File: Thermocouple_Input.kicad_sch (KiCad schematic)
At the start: 9 parts, among them J7 K-TYPE THERMOCOUPLE, U11 MAX31856

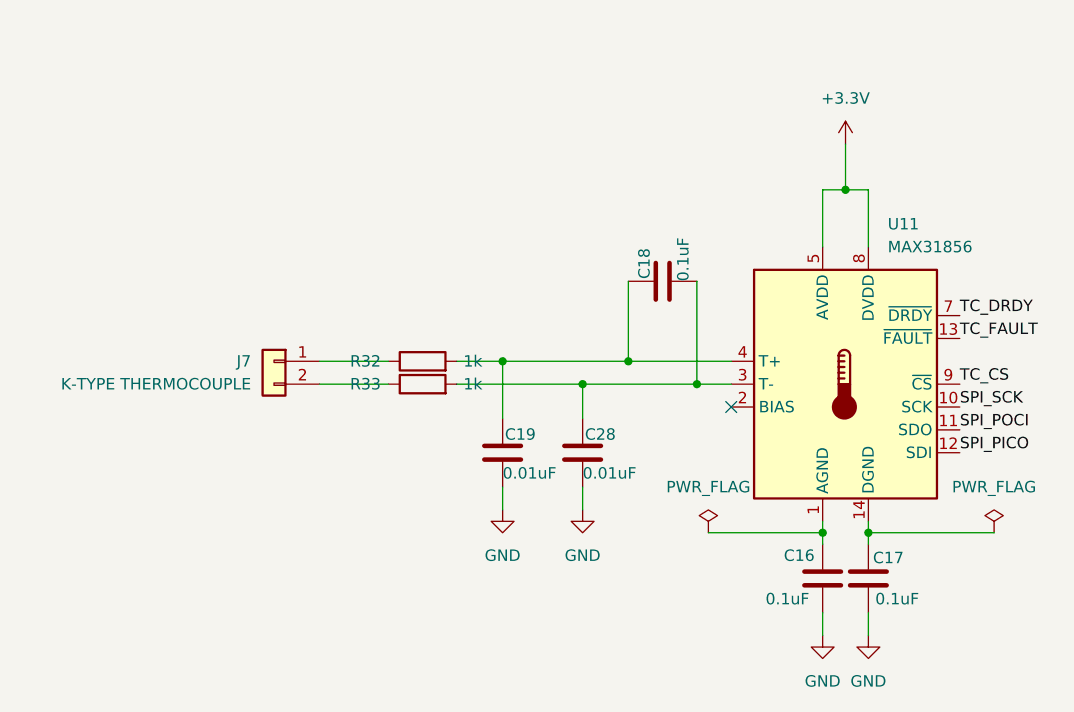
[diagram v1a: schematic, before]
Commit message: Grayson changes 9/11/26
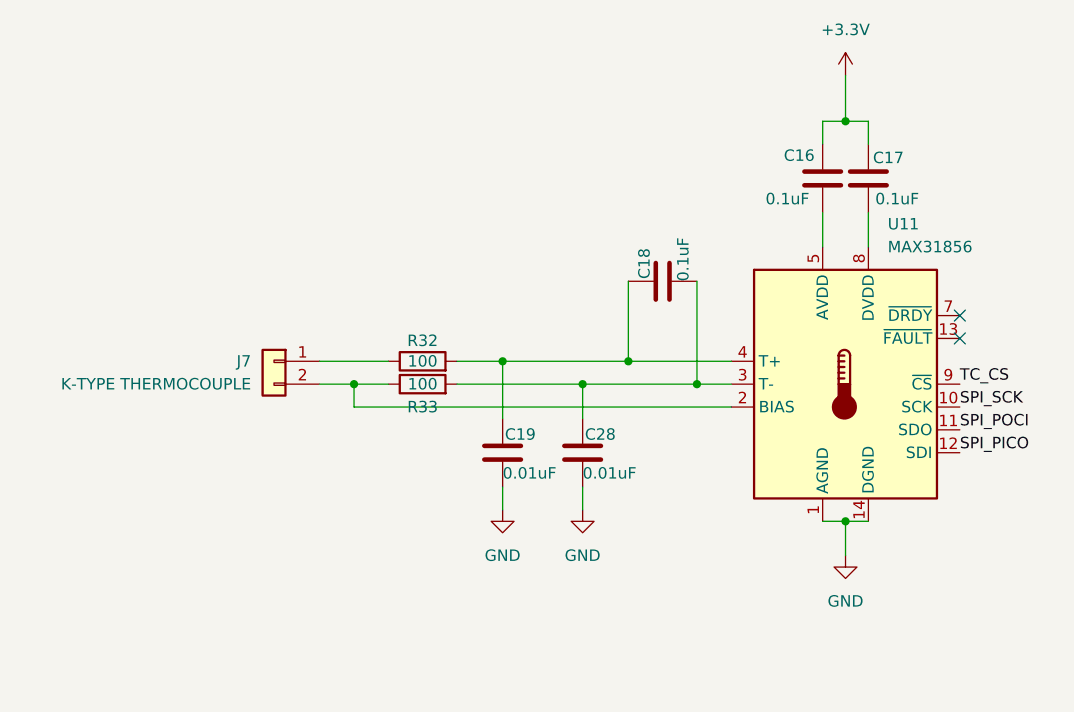
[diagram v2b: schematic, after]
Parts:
- R32, R33: value 1k -> 100
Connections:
- net +3.3V: now also C16.1, C17.1; no longer U11.5 (AVDD), U11.8 (DVDD)
- net GND: now also U11.1 (AGND), U11.14 (DGND); no longer C16.2, C17.2
- net at U11.2 (BIAS): now also J7.2 (Pin_2), R33.1
- net TC_DRDY: no longer names the net of U11.7 (~{DRDY})
- net TC_FAULT: no longer names the net of U11.13 (~{FAULT})
- new net: C16.2, U11.5 (AVDD)
- new net: C17.2, U11.8 (DVDD)
- no-connect marks 1 -> 2
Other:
- moved on the sheet: C16, C17
